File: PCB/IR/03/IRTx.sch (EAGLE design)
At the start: 13 parts

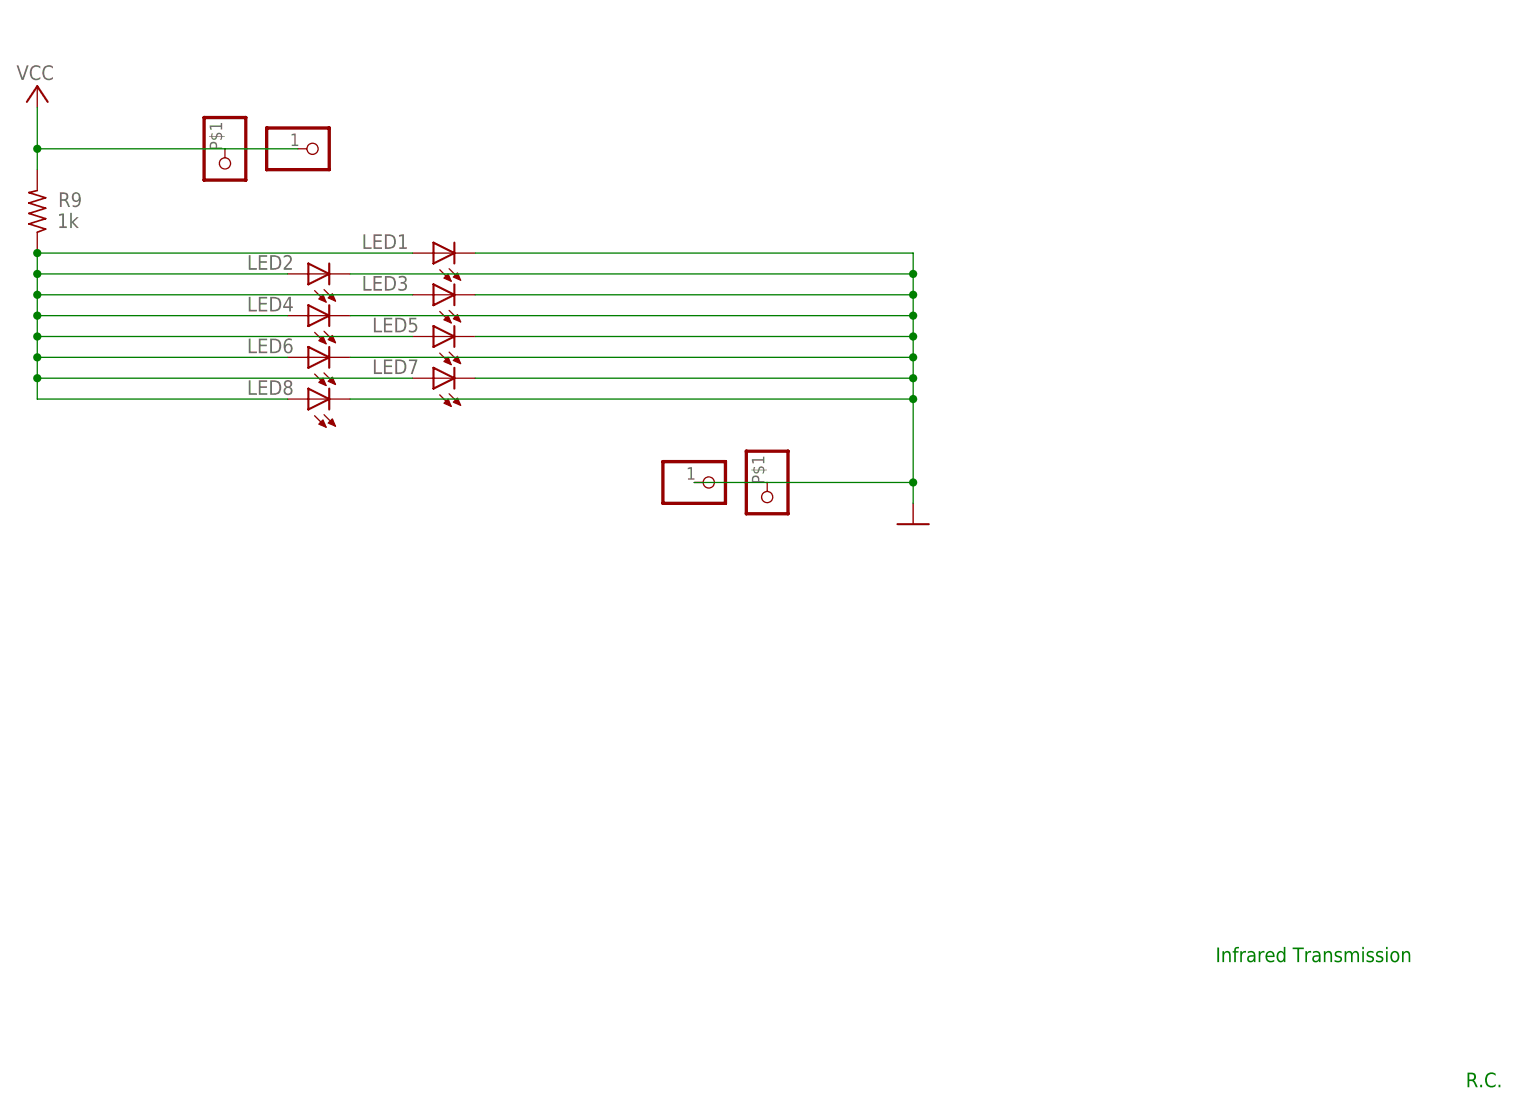
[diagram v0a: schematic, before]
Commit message: modified IR-TX
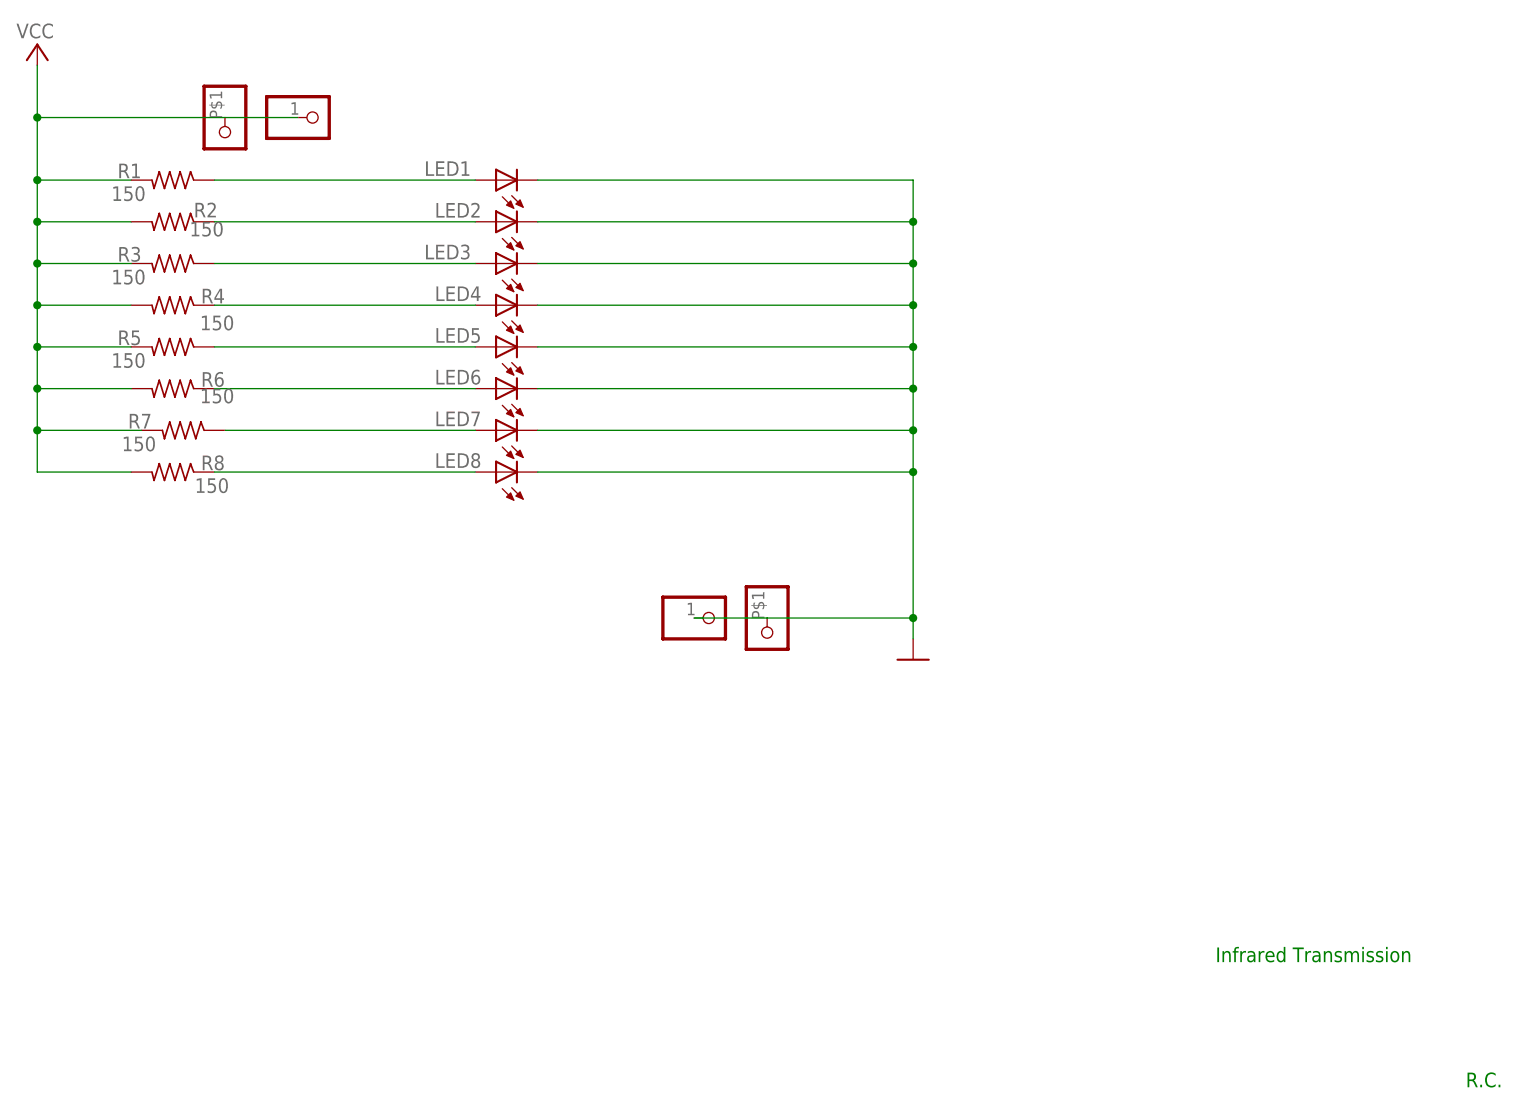
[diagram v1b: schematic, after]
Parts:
- removed R9: 1k, adafruit:R-US_0207/10
- added R1, R2, R3, R4, R5, R6, R7, R8: 150, adafruit:R-US_0207/10
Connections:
- new net N$2: LED1.A, R1.1
- new net N$3: LED3.A, R3.1
- new net N$4: LED4.A, R4.1
- new net N$5: LED5.A, R5.1
- new net N$6: LED6.A, R6.1
- new net N$7: LED7.A, R7.1
- new net N$8: LED8.A, R8.1
- net N$1: now also R2.1; no longer LED1.A, LED3.A, LED4.A, LED5.A, LED6.A, LED7.A, LED8.A, R9.1
- net VCC: now also R1.2, R2.2, R3.2, R4.2, R5.2, R6.2, R7.2, R8.2; no longer R9.2
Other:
- moved on the sheet: LED1, LED2, LED3, LED4, LED5, LED6, LED7, LED8
